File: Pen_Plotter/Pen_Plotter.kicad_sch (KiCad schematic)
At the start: 39 parts, among them J1 USB_Type-C_Breakout, J2 PinHeader_01x05_P2.54mm_Verti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, J3 PinHeader_01x05_P2.54mm_Verti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, J4 Screw_Terminal_01x02_P3.5mm, J5 PinHeader_01x02_P2.54mm_Verti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, J6 PinHeader_01x02_P2.54mm_Verti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, J7 PinHeader_01x03_P2.54mm_Verti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, Q1 Transistor_MOSFET_NCh_SOT23, Q2 Transistor_MOSFET_NCh_SOT23, SW1 Switch_Tactile_Omron, SW2 Switch_Tactile_Omron, U1 ESP32-WROOM-32E, U2 Regulator_Linear_3.3V_1A_Diod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, U3 CH340C, U4 ULN2803

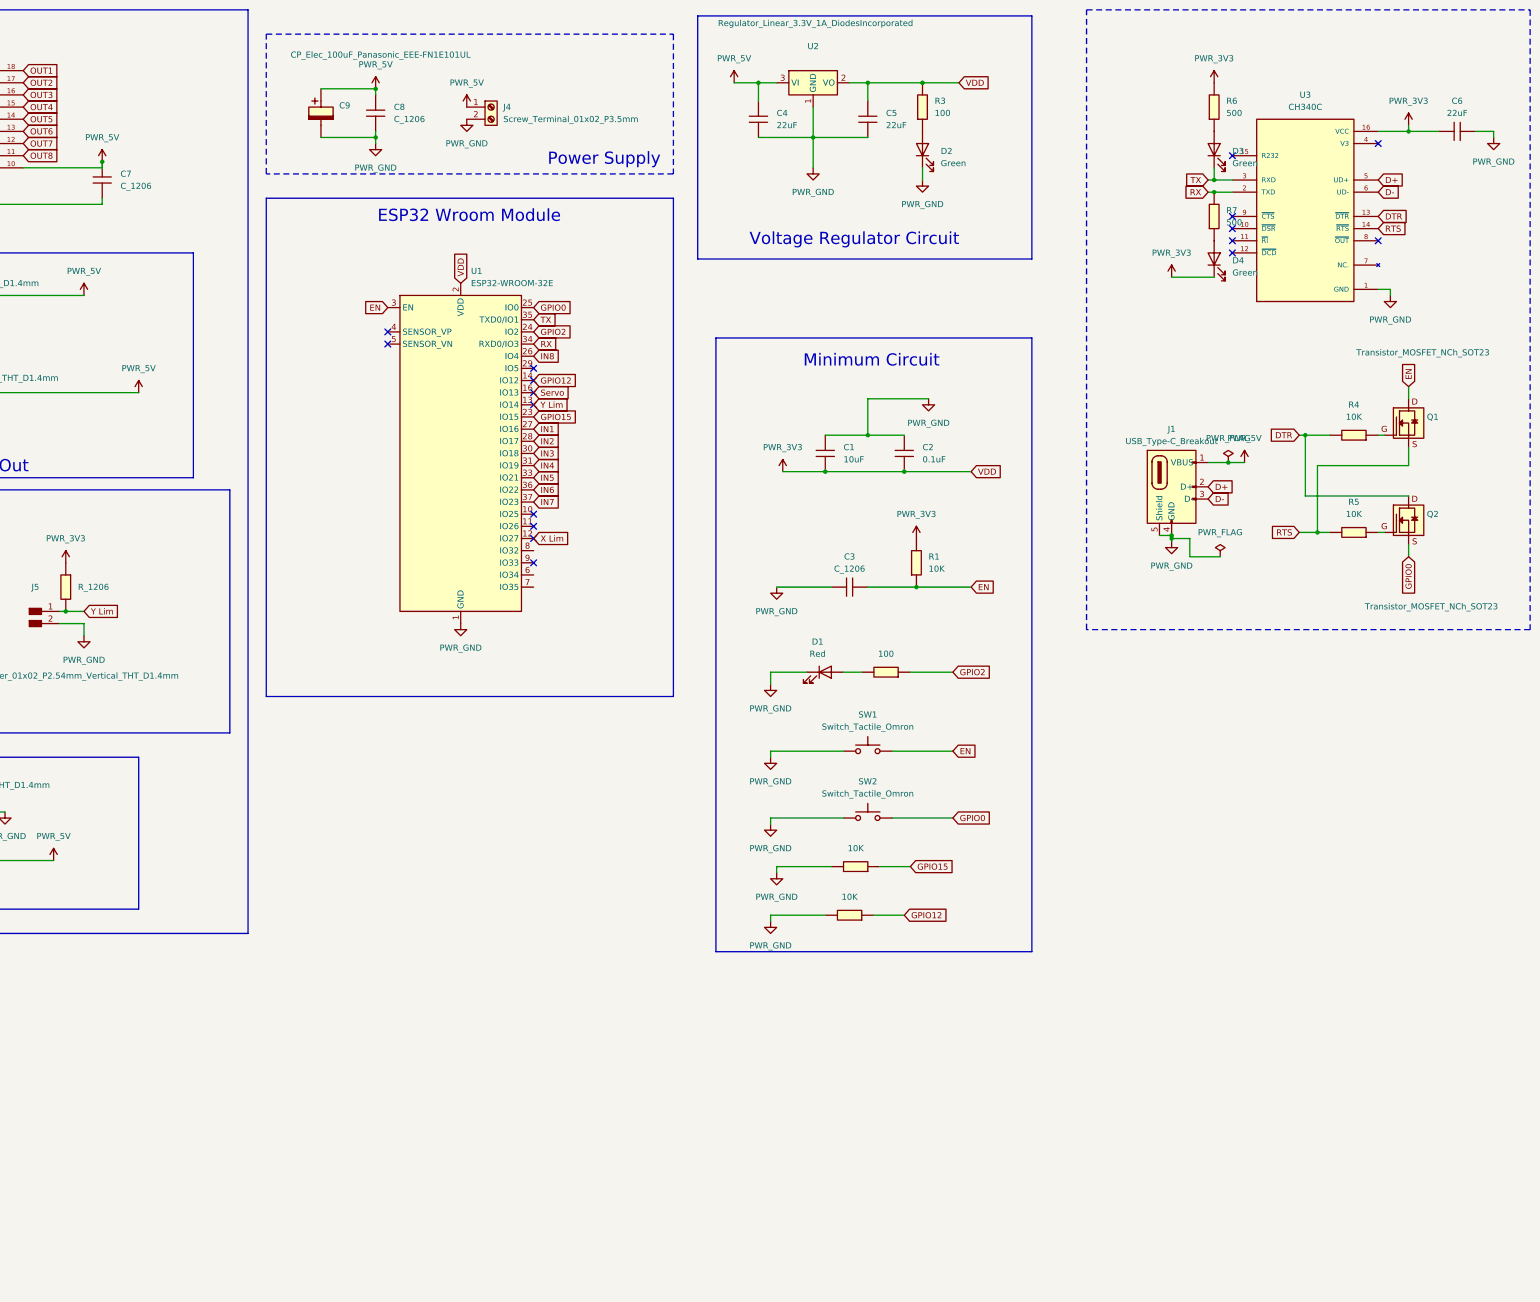
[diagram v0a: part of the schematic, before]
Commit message: PCB for ESP UCap
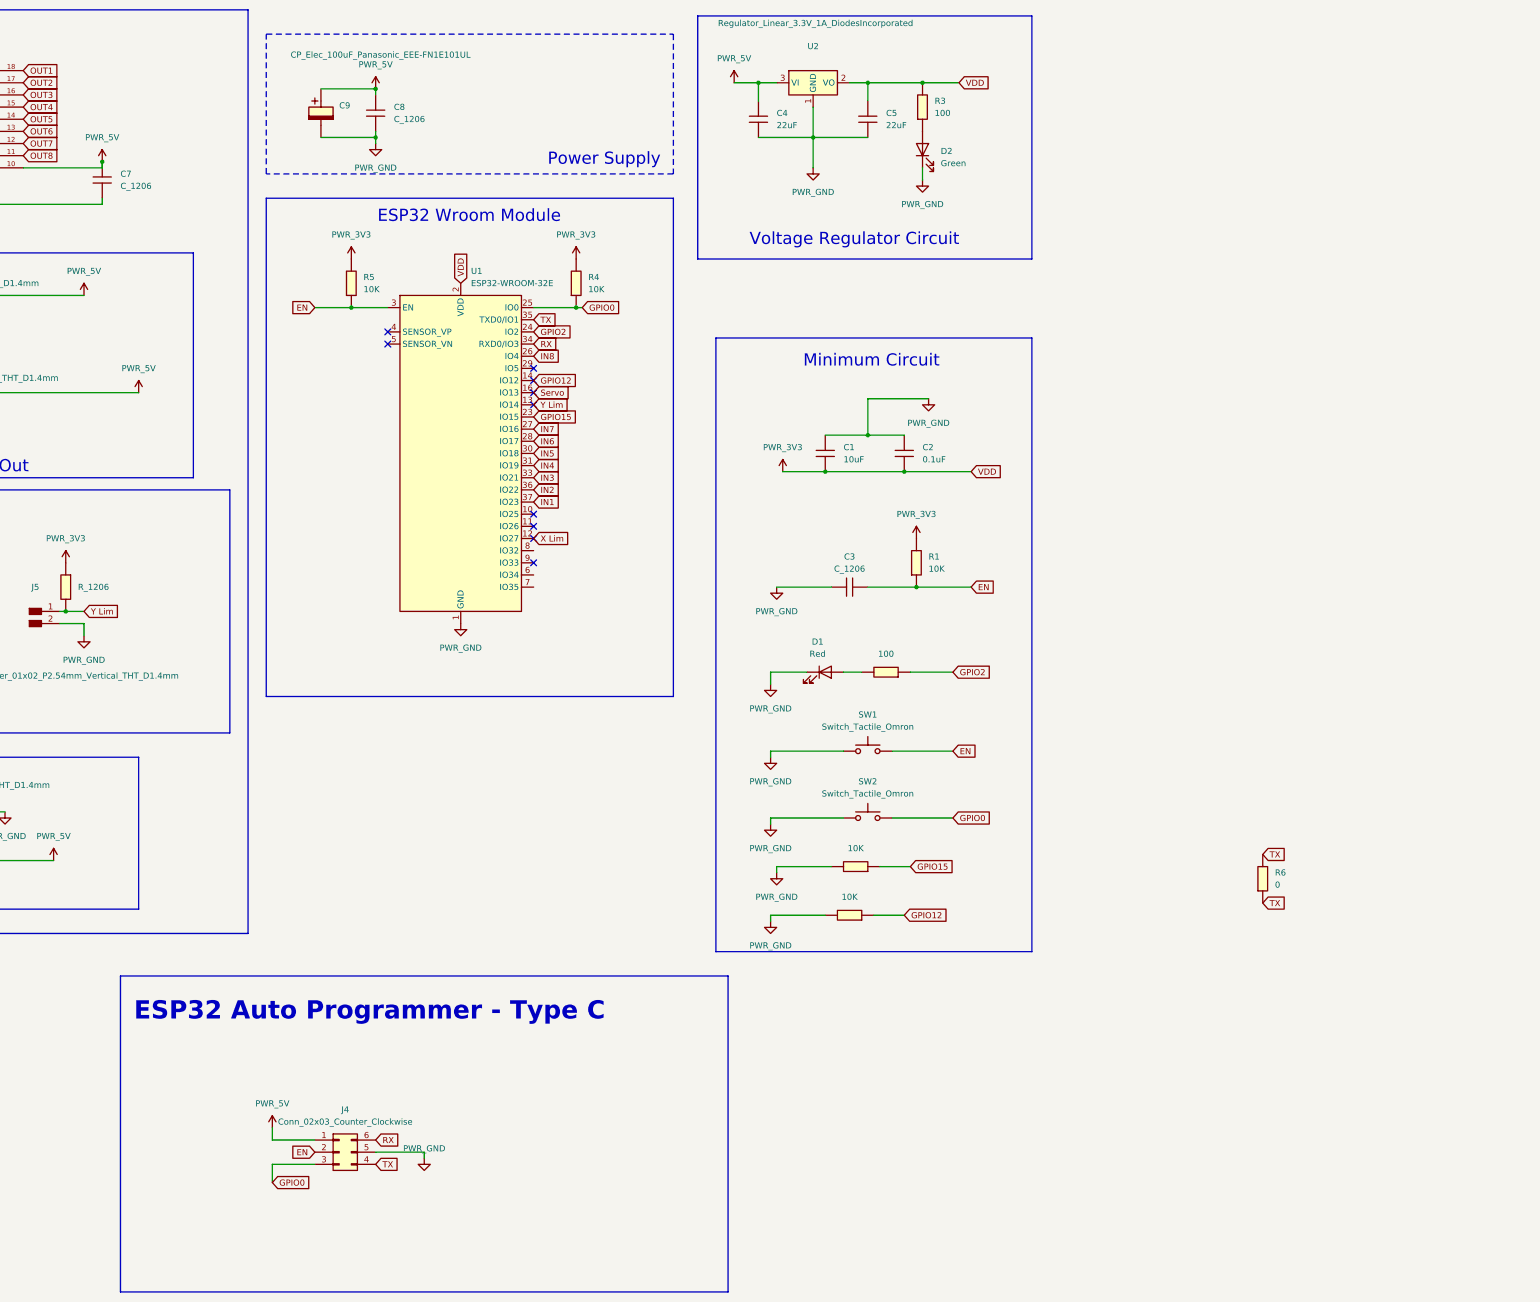
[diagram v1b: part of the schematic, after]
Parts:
- removed C6: 22uF, fab:C_1206, symbol fab:C_1206
- removed D3, D4: Green, fab:LED_1206, symbol fab:LED_1206
- removed J1: USB_Type-C_Breakout, Proshplay Type C:ProshPlay-Type-C-breakout-board, symbol ProshPlay:ProshPlay-Type-C-breakout-board
- removed J4: Screw_Terminal_01x02_P3.5mm, fab:TerminalBlock_OnShore_1x02_P3.50mm_Horizontal, symbol fab:Screw_Terminal_01x02_P3.5mm
- removed Q1, Q2: Transistor_MOSFET_NCh_SOT23, fab:SOT-23-3, symbol fab:Transistor_MOSFET_NCh_SOT23
- removed R7: 500, fab:R_1206, symbol fab:R_1206
- removed U3: CH340C, CH340C:SOIC127P600X180-16N, symbol CH340C:CH340C
- added J4: Conn_02x03_Counter_Clockwise, Connector_PinHeader_2.54mm:PinHeader_2x03_P2.54mm_Horizontal, symbol Connector_Generic:Conn_02x03_Counter_Clockwise
- R6: value 500 -> 0
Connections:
- net DTR is gone; now on net PWR_3V3: R4.1
- net RTS is gone; now on net PWR_3V3: R5.1
- net EN: now also R5.2, J4.2 (Pin_2)
- net GPIO0: now also R4.2, J4.3 (Pin_3)
- net IN1: now also U1.37 (IO23); no longer U1.27 (IO16)
- net IN2: now also U1.36 (IO22); no longer U1.28 (IO17)
- net IN3: now also U1.33 (IO21); no longer U1.30 (IO18)
- net IN5: now also U1.30 (IO18); no longer U1.33 (IO21)
- net IN6: now also U1.28 (IO17); no longer U1.36 (IO22)
- net IN7: now also U1.27 (IO16); no longer U1.37 (IO23)
- net PWR_3V3: no longer R6.1
- net PWR_5V: now also J4.1 (Pin_1)
- net PWR_GND: now also J4.5 (Pin_5)
- net RX: now also J4.6 (Pin_6)
- net TX: now also R6.1, R6.2, J4.4 (Pin_4)
- no-connect marks 17 -> 10
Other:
- note added: "ESP32 Auto Programmer - Type C"
